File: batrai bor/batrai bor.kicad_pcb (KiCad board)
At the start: 2 copper layers, 47 x 33 mm, 15 parts, among them J10 +, J11 +, J12 -, J13 -, J2 Molex, J3 2, J4 3, J5 4, J6 5, J8 1, J9 6

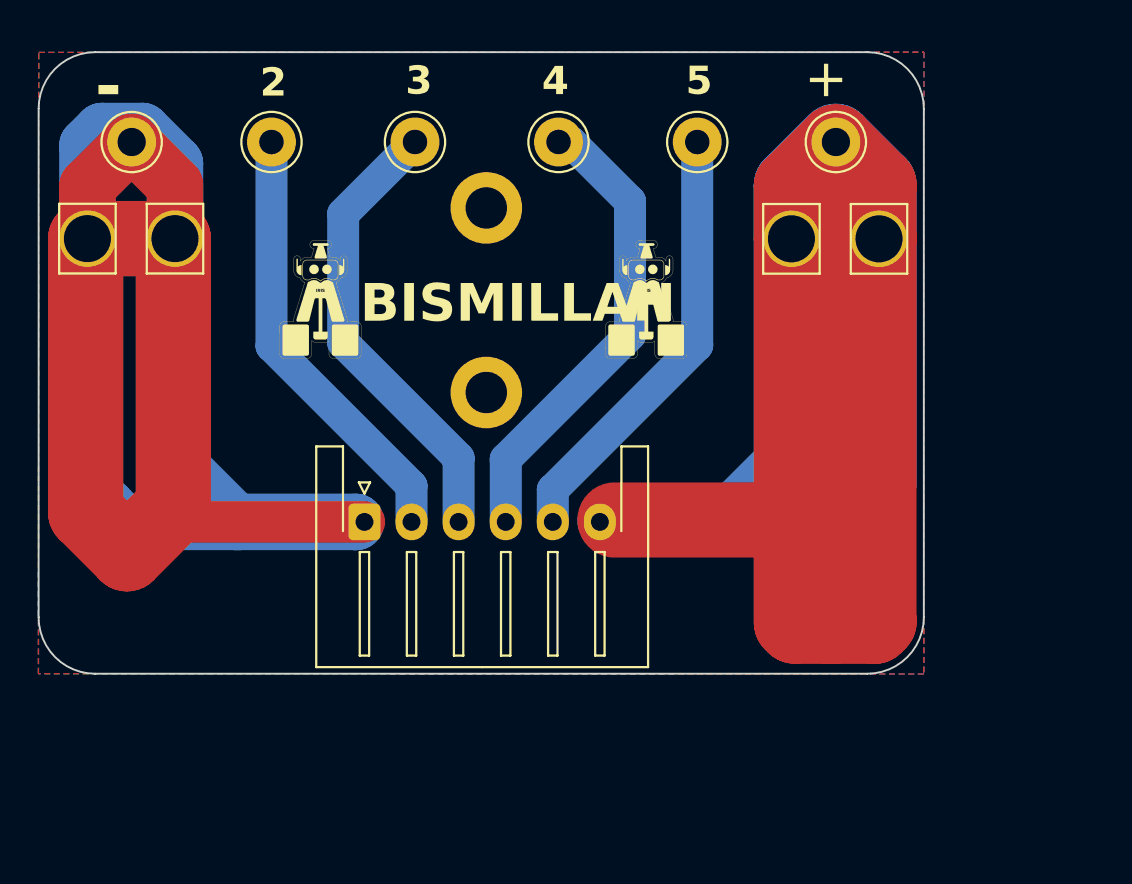
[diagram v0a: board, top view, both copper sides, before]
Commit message: V.4.1
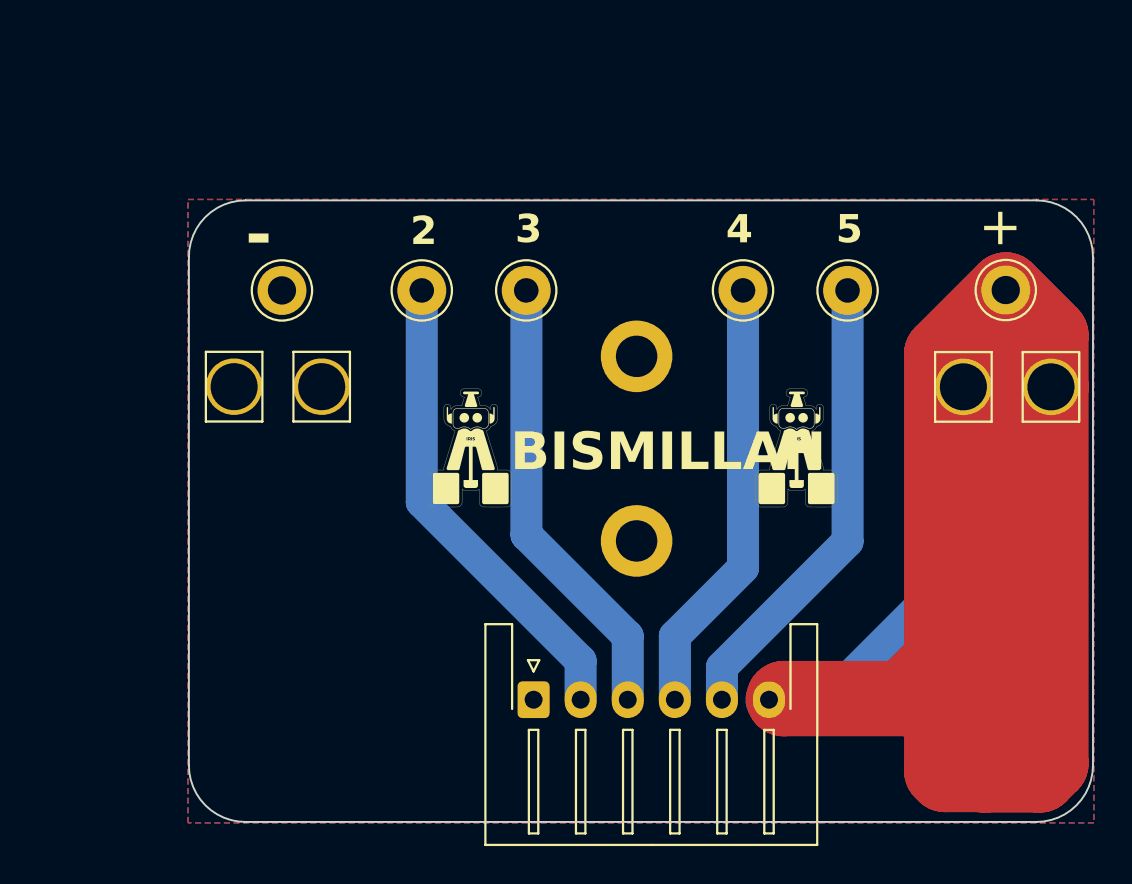
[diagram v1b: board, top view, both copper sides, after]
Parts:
- moved J2 13.0 mm to (38.3, 46.4)
- moved J5 12.6 mm to (49.4, 24.6)
- moved J10 12.0 mm to (65.8, 29.8)
- moved J11 12.0 mm to (61.1, 29.8)
- moved J9 12.0 mm to (63.4, 24.6)
- moved G*** 11.2 mm to (52.2, 33.0)
- moved J6 11.2 mm to (55.0, 24.6)
- moved H2 11.2 mm to (43.8, 38.0)
- moved J3 11.2 mm to (32.3, 24.6)
- moved J8 11.2 mm to (24.9, 24.6)
- moved G*** 11.2 mm to (34.9, 33.0)
- moved H1 11.2 mm to (43.8, 28.1)
- moved J12 11.1 mm to (27.0, 29.8)
- moved J13 11.1 mm to (22.4, 29.8)
- moved J4 9.85 mm to (37.9, 24.6)
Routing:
- net /-: track 128.1 -> 0.00 mm
- net /+: track 198.6 -> 193.0 mm
- net Net-(J2-Pin_2): track 23.3 -> 25.2 mm
- net Net-(J2-Pin_4): track 24.9 -> 23.2 mm
- net Net-(J2-Pin_5): track 23.3 -> 24.5 mm
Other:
- board size 47 x 33 mm -> 48 x 33 mm
